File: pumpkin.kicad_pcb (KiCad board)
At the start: 4 copper layers, 51 x 45.1 mm, 24 parts, among them J1 MK-12C02

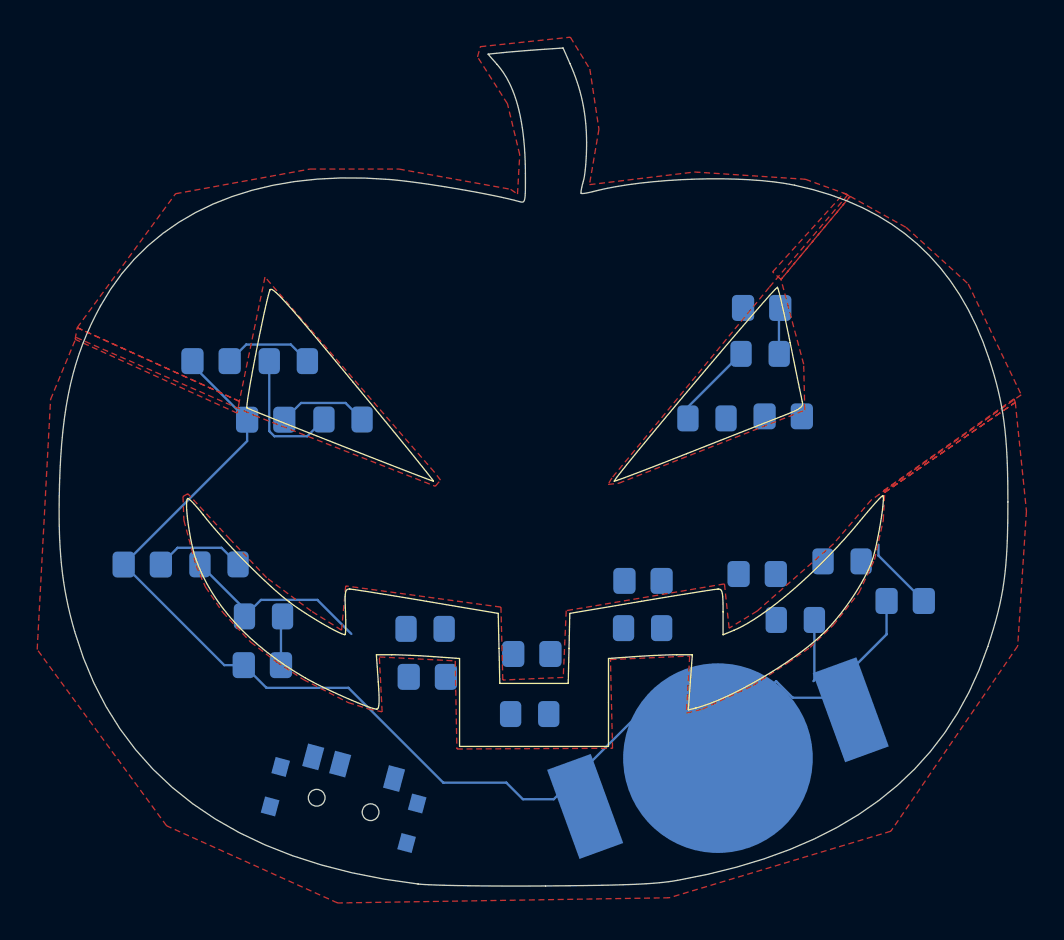
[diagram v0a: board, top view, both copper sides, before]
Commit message: finished tracks
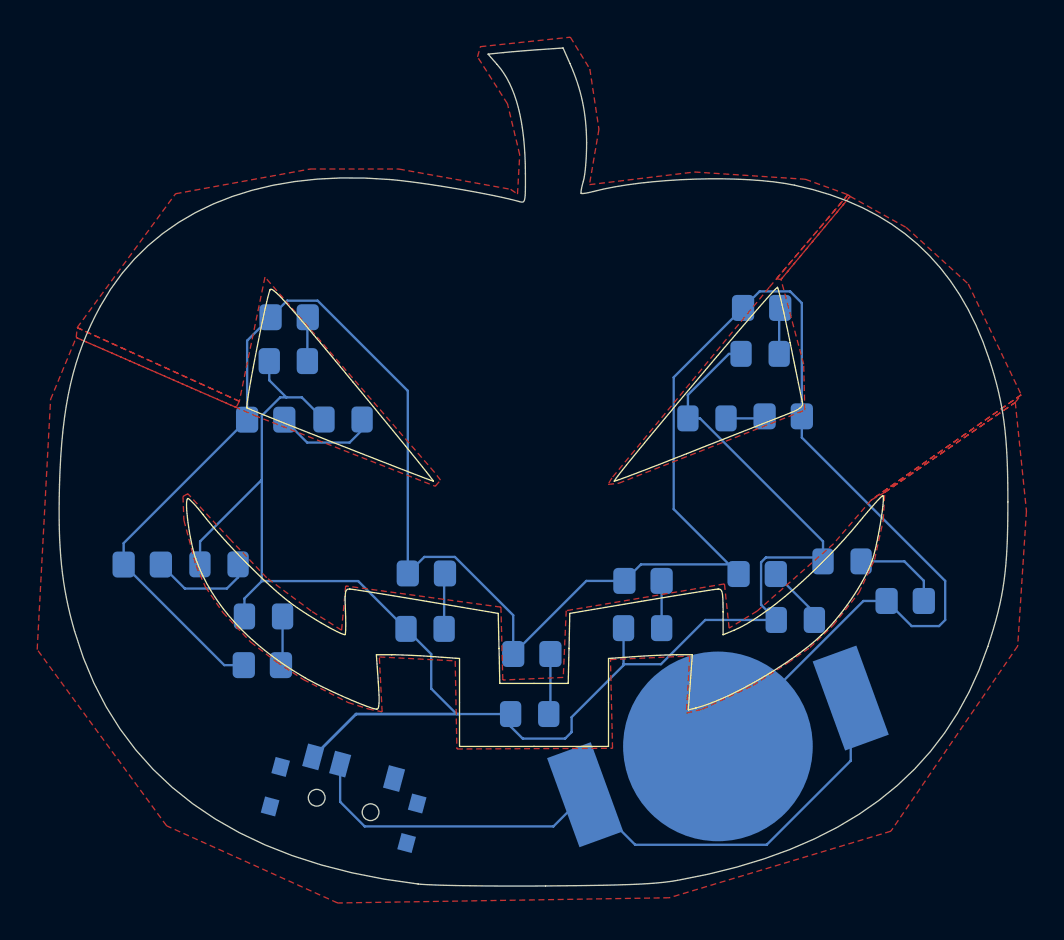
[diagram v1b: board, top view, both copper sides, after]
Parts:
- moved R7 5.56 mm to (139.3, 100.8)
- moved R1 4.82 mm to (132.0, 87.0)
- moved BT1 0.63 mm to (155.0, 110.1)
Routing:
- net Net-(D1-A): track 22.5 -> 93.3 mm
- net GND: track 68.1 -> 126.1 mm
- net Net-(BT1-+): track 0.00 -> 37.1 mm
- net Net-(D8-K): track 0.00 -> 3.27 mm
- net Net-(D7-K): track 0.00 -> 3.00 mm
- net Net-(D1-K): track 4.92 -> 2.37 mm
- net Net-(D9-K): track 0.00 -> 2.54 mm
- net Net-(D4-K): track 0.00 -> 2.12 mm
- net Net-(D11-K): track 4.04 -> 4.89 mm
- net Net-(D5-K): track 4.89 -> 5.63 mm
- net Net-(D3-K): track 4.92 -> 5.54 mm
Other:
- rule pad_to_mask_clearance: 0 -> 0.0508
- rule solder_mask_min_width: 0.12 -> 0.25
